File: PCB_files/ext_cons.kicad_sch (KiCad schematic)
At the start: 19 parts, among them J1 FFC2B28-40-G, J2 CANbus, J3 uUSB, J4 CM4-A, J6 CM4-B, J7 HDMI_ribbon, SW7 nBoot, U2 FSUSB42MUX, U4 TPD8S009DSMR, U5 TPD8S009DSMR, U6 TPD2EUSB30

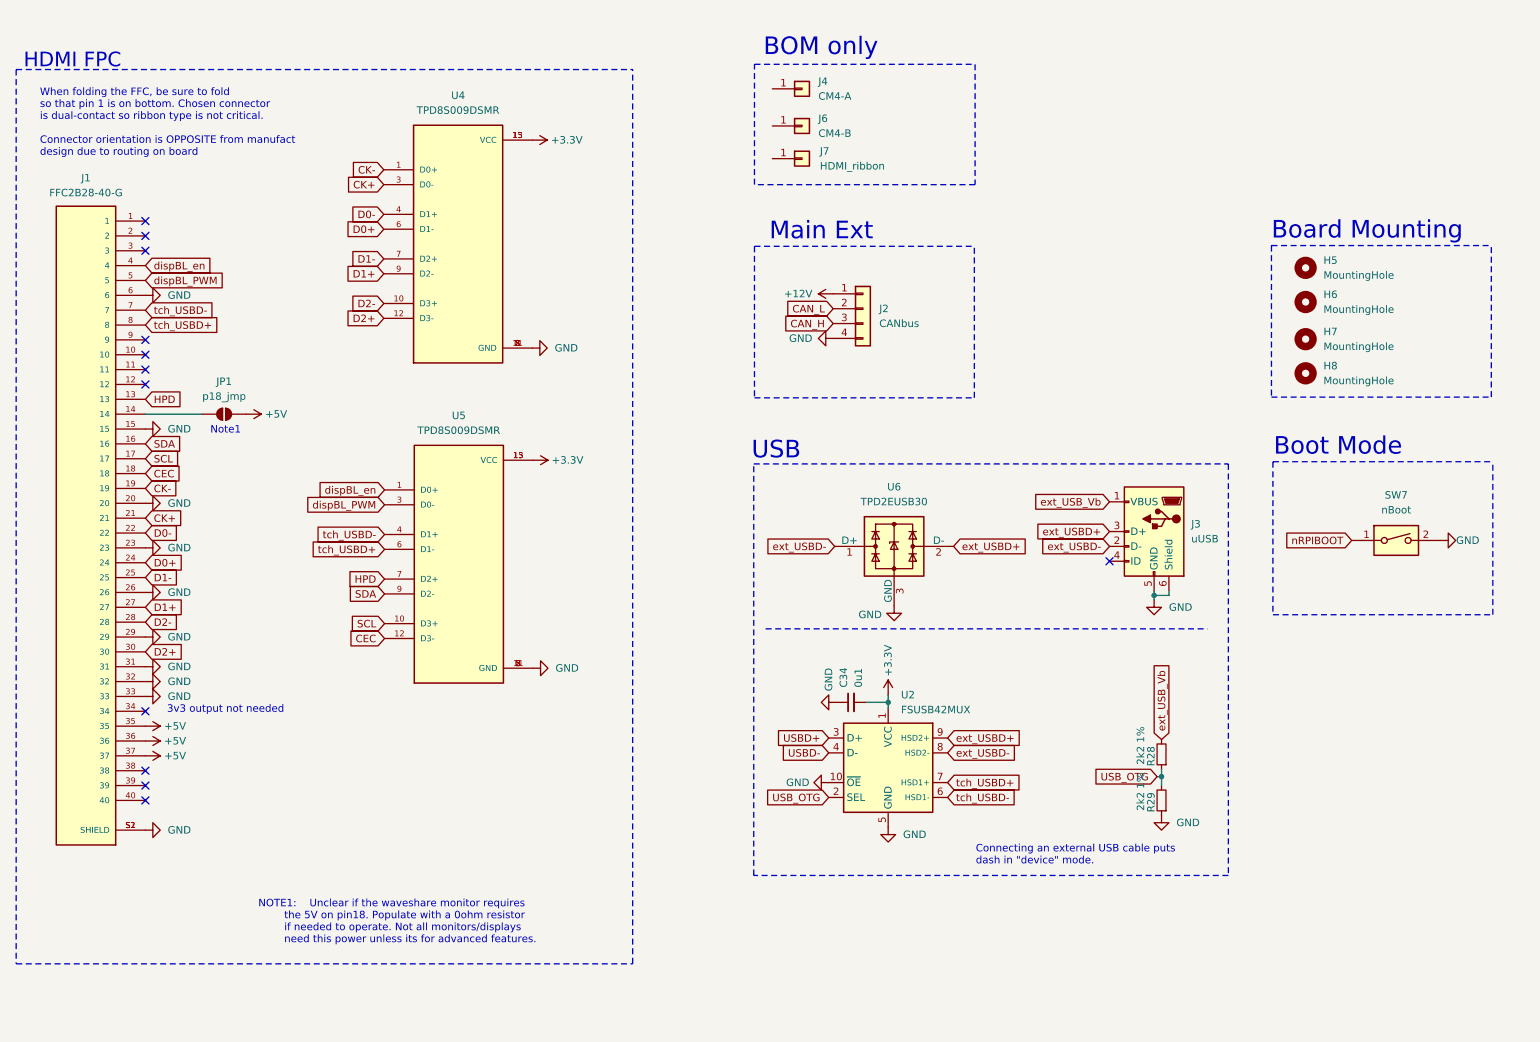
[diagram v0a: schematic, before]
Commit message: Rev2a initial upload
PCB files
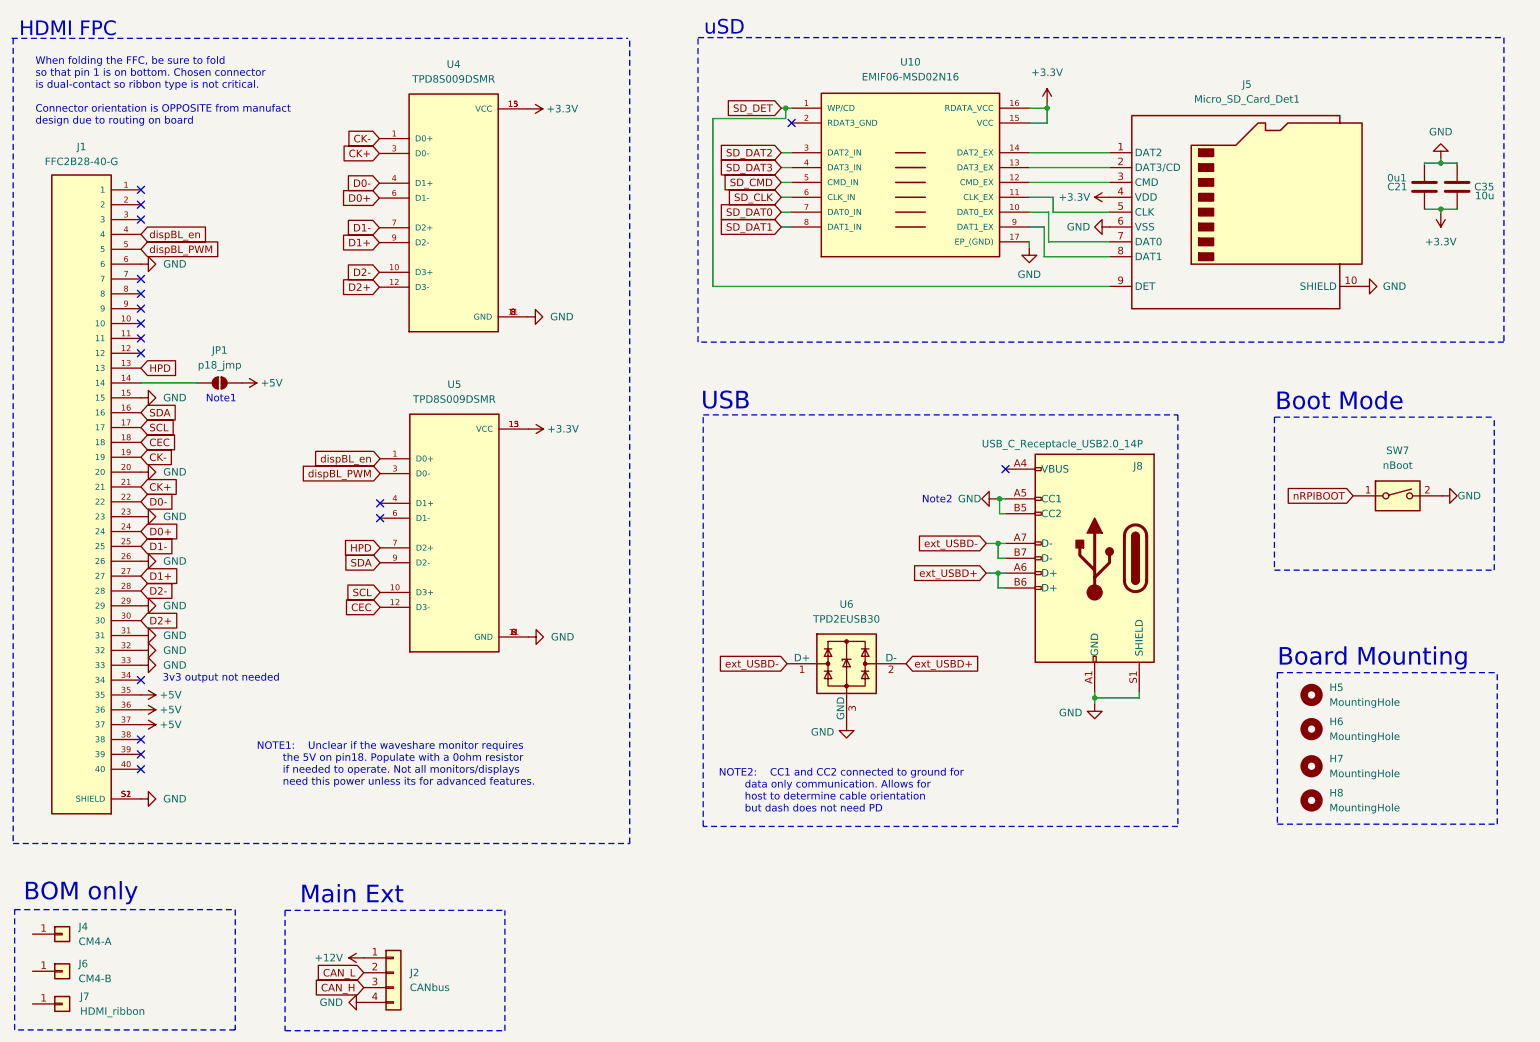
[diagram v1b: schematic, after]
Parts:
- removed C34: 0u1, Capacitor_SMD:C_0805_2012Metric, symbol Device:C_Small
- removed J3: uUSB, user:GCT_USB3140-30-0170-1-C_REVE1, symbol Connector:USB_B_Micro
- removed R28, R29: 2k2 1%, Resistor_SMD:R_0805_2012Metric, symbol Device:R_Small
- removed U2: FSUSB42MUX, Package_SO:MSOP-10_3x3mm_P0.5mm, symbol Interface_USB:FSUSB42MUX
- added C21: 0u1, Capacitor_SMD:C_0805_2012Metric, symbol Device:C
- added C35: 10u, Capacitor_SMD:C_0805_2012Metric, symbol Device:C
- added J5: Micro_SD_Card_Det1, Connector_Card:microSD_HC_Hirose_DM3AT-SF-PEJM5, symbol Connector:Micro_SD_Card_Det1
- added J8: USB_C_Receptacle_USB2.0_14P, Connector_USB:USB_C_Receptacle_GCT_USB4115-03-C, symbol Connector:USB_C_Receptacle_USB2.0_14P
- added U10: EMIF06-MSD02N16, user:EMIF06MSD02N16, symbol user:EMIF06-MSD02N16
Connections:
- net +3.3V: now also C21.1, C35.2, J5.4 (VDD), U10.15 (VCC), U10.16 (RDATA_VCC)
- net GND: now also C21.2, C35.1, J5.10 (SHIELD), J5.6 (VSS), J8.A1 (GND), J8.A12 (GND), J8.A5 (CC1), J8.B1 (GND), J8.B12 (GND), J8.B5 (CC2), J8.S1 (SHIELD), U10.17 (EP_(GND))
- net ext_USBD+: now also J8.A6 (D+), J8.B6 (D+)
- net ext_USBD-: now also J8.A7 (D-), J8.B7 (D-)
- net tch_USBD+: no longer names the net of J1.8
- net tch_USBD+: no longer U5.6 (D1-)
- net tch_USBD-: no longer names the net of J1.7
- net tch_USBD-: no longer U5.4 (D1+)
- new net: J8.A4 (VBUS), J8.A9 (VBUS), J8.B4 (VBUS), J8.B9 (VBUS)
- new net: J5.1 (DAT2), U10.14 (DAT2_EX)
- new net: J5.2 (DAT3/CD), U10.13 (DAT3_EX)
- new net: J5.3 (CMD), U10.12 (CMD_EX)
- new net: J5.5 (CLK), U10.11 (CLK_EX)
- new net: J5.7 (DAT0), U10.10 (DAT0_EX)
- new net: J5.8 (DAT1), U10.9 (DAT1_EX)
- new net SD_CLK: U10.6 (CLK_IN)
- new net SD_CMD: U10.5 (CMD_IN)
- new net SD_DAT0: U10.7 (DAT0_IN)
- new net SD_DAT1: U10.8 (DAT1_IN)
- new net SD_DAT2: U10.3 (DAT2_IN)
- new net SD_DAT3: U10.4 (DAT3_IN)
- new net SD_DET: J5.9 (DET), U10.1 (WP/CD)
- no-connect marks 12 -> 17
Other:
- note added: "NOTE2: CC1 and CC2 connected to ground for data only communication. Allows for host to determine cable orientation but dash does not need PD"
- note added: "Note2"
- note added: "uSD"
- note removed: "Connecting an external USB cable puts dash in "device" mode."
- moved on the sheet: H5, H6, H7, H8, J1, J2, J4, J6, J7, JP1, SW7, U4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
